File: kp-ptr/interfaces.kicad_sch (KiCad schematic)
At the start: 2 parts

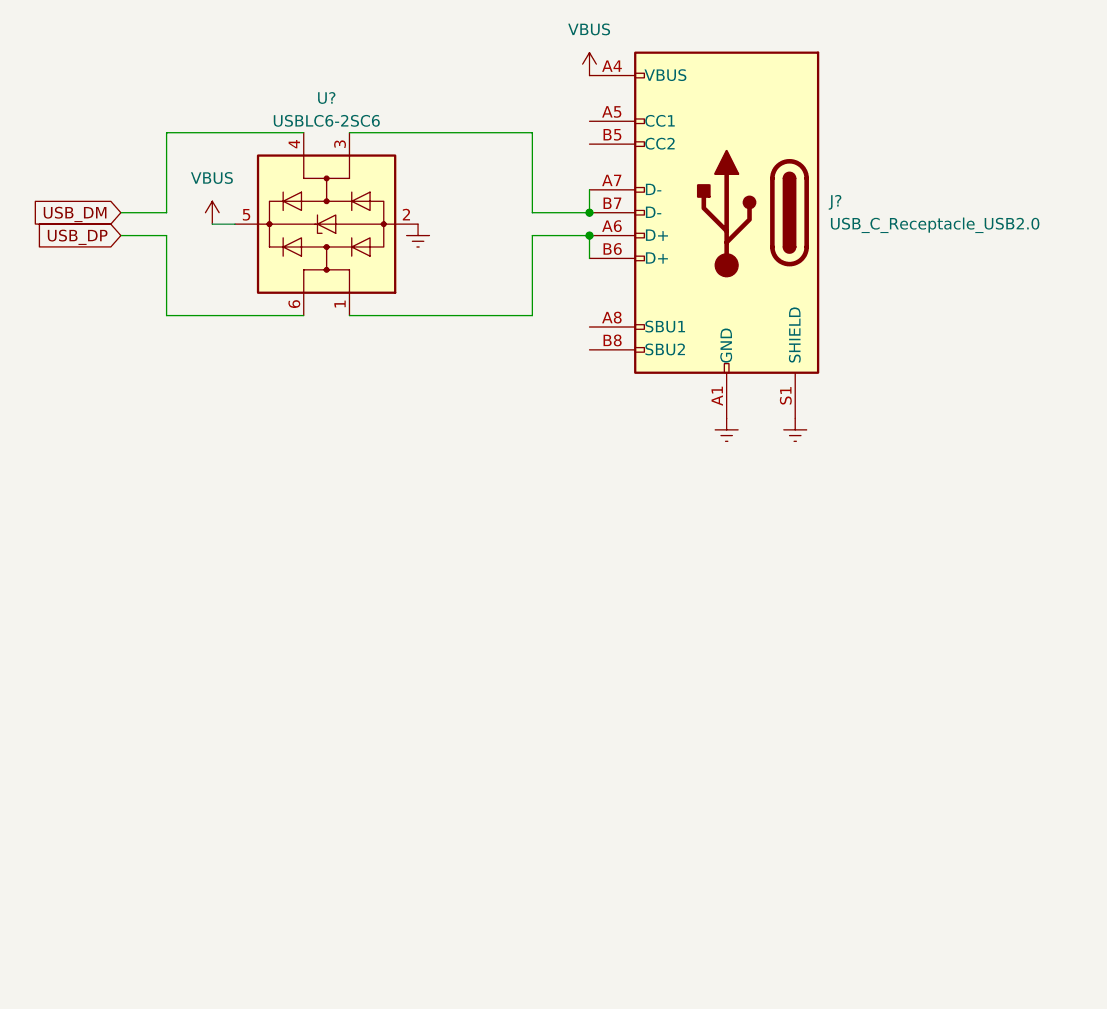
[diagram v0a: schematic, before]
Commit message: LIS + SDCARD Signed-off-by: kretu <krecik@gmail.com>
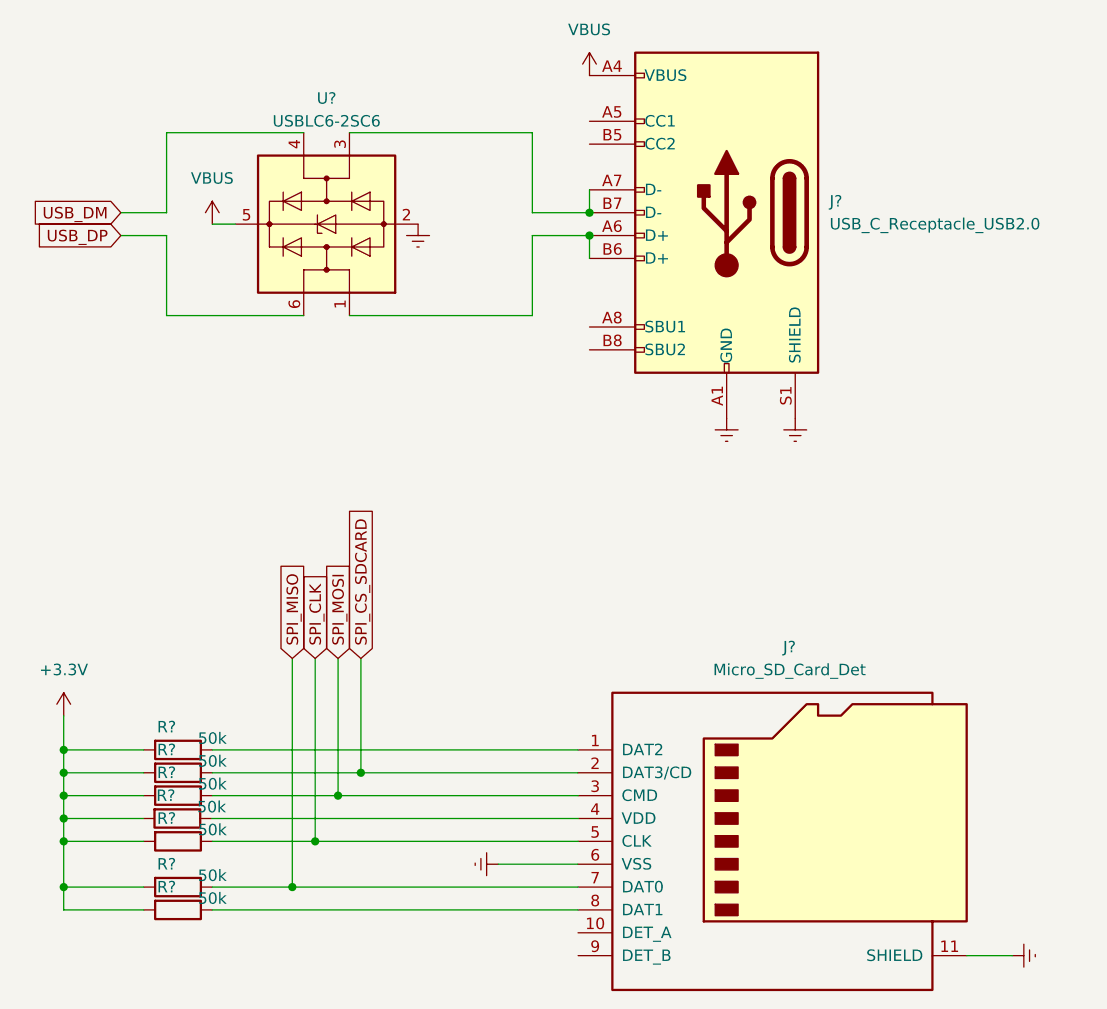
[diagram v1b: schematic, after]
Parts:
- added J?: Micro_SD_Card_Det, symbol Connector:Micro_SD_Card_Det
- added R? (x7): 50k, symbol Device:R
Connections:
- net Earth: now also J?.11 (SHIELD), J?.6 (VSS)
- new net: J?.4 (VDD), R?.1
- new net: J?.8 (DAT1), R?.1
- new net: J?.1 (DAT2), R?.1
- new net +3V3: R?.2, R?.2, R?.2, R?.2, R?.2, R?.2, R?.2
- new net SPI_CLK: J?.5 (CLK), R?.1
- new net SPI_CS_SDCARD: J?.2 (DAT3/CD), R?.1
- new net SPI_MISO: J?.7 (DAT0), R?.1
- new net SPI_MOSI: J?.3 (CMD), R?.1
